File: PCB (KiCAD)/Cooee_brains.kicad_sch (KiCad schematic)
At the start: 36 parts, among them J1 USB4105-GF-A, J2 Conn_Coaxial, J3 503398-1892, J4 Conn_01x14_Socket, J5 Conn_01x02_Pin, J6 Conn_Coaxial, J7 Conn_01x04_Pin, J9 Conn_01x05_Socket, SW1 Prog, SW2 Reset, U1 AMS1117-3.3, U2 ESP32-S3-WROOM-1-N8, U3 MAX98357AETE_T, U6 INTERFACE-CP2102-GMR_QFN28_, U8 RA-01H

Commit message: more PCB work on the motherboard
more PCB work on the motherboard
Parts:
- added C5, C9: 4.7uF, Capacitor_SMD:C_0805_2012Metric, symbol Device:C_Small
- added C6, C8: 100nF, Capacitor_SMD:C_0805_2012Metric, symbol Device:C_Small
- added C7: 1uF, Capacitor_SMD:C_0805_2012Metric, symbol Device:C_Small
- added D1: D, Diode_SMD:D_0805_2012Metric_Pad1.15x1.40mm_HandSolder, symbol Device:D
- added H3: MountingHole_Pad_MP, MountingHole:MountingHole_3.2mm_M3_DIN965_Pad_TopBottom, symbol Mechanical:MountingHole_Pad_MP
- added JP1: SolderJumper_2_Open, Jumper:SolderJumper-2_P1.3mm_Open_RoundedPad1.0x1.5mm, symbol Jumper:SolderJumper_2_Open
- added R11, R12, R13, R14, R8: 10kΩ, Capacitor_SMD:C_0805_2012Metric_Pad1.18x1.45mm_HandSolder, symbol stormduino-Rev2-rescue:R-Device
- U5: value ~ -> M210Z
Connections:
- net BigSD_MISO is gone; now on net SHARED_MISO: J7.2 (Pin_2)
- net BigSD_MOSI is gone; now on net SHARED_MOSI: J7.3 (Pin_3)
- net BigSD_SCK is gone; now on net SHARED_CLCK: J7.1 (Pin_1)
- net SD_CLK is gone; now on net SHARED_CLCK: J3.5 (CLK)
- net SD_DAT0 is gone; now on net SHARED_MISO: J3.7 (DAT0)
- net 3.3V: now also J3.4 (VDD), MK1.7 (VDD), U5.14 (Vcc_RF), U5.8 (VCC), U6.6 (VDD), C8.2, C9.1, R11.1, R12.1
- net 5V: now also U6.7 (REGIN), U6.8 (VBUS), C6.1, C7.1, D1.2 (A); no longer C1.2, U1.3 (VI)
- net Batt+: now also C1.2, U1.3 (VI), D1.1 (K)
- net GND: now also C5.1, C6.2, C7.2, C8.1, C9.2, H3.MP, R13.1, R14.1, R8.1
- net KEEB_SCL: now also U2.10 (IO17); no longer U2.15 (IO3)
- net LoRa_Select: now also U2.25 (IO48); no longer U2.16 (IO46)
- net SHARED_CLCK: now also J4.10 (Pin_10), U8.12 (SCK)
- net SHARED_MISO: now also J4.13 (Pin_13), U8.13 (MISO)
- net SHARED_MOSI: now also J3.3 (CMD), J4.12 (Pin_12), U8.14 (MOSI)
- net SPEAKER+: now also J5.2 (Pin_2); no longer J5.1 (Pin_1)
- net SPEAKER-: now also J5.1 (Pin_1); no longer J5.2 (Pin_2)
- net T_CS: now also U2.8 (IO15); no longer U2.21 (IO13)
- net USB_D+: no longer U6.4 (D+)
- net USB_D-: no longer U6.5 (D-)
- net USB_DN: now also U6.5 (D-); no longer U2.13 (IO19)
- net USB_DP: now also U6.4 (D+); no longer U2.14 (IO20)
- net MIC_BCLK: now reaches U2.11 (IO18)
- net MIC_BCLK: now also MK1.1 (SCK)
- net MIC_EN: now reaches U2.23 (IO21)
- net MIC_EN: now also MK1.8 (CHIPEN)
- net GPS_RST: now reaches U2.32 (IO39)
- net GPS_RST: now also U5.9 (RST)
- net GPS_On/OFF: now reaches U2.33 (IO40)
- net GPS_On/OFF: now also U5.5 (On/Off)
- net GPS_SlaveIn: now reaches U2.34 (IO41)
- net GPS_SlaveIn: now also U5.3 (GPS_RxData)
- net GPS_SlaveOut: now reaches U2.35 (IO42)
- net GPS_SlaveOut: now also U5.2 (GPS_TxData)
- net Interface_Tx: now reaches U2.36 (RXD0)
- net Interface_Tx: now also U6.26 (TXD)
- net Interface_Rx: now reaches U2.37 (TXD0)
- net Interface_Rx: now also U6.25 (RXD)
- net SPKR_DIN: now reaches U3.1 (DIN)
- net SPKR_DIN: now also U2.21 (IO13)
- net SPKR_LRCK: now reaches U3.14 (LRCLK)
- net SPKR_LRCK: now also U2.22 (IO14)
- net SPKR_BCLK: now reaches U3.16 (BCLK)
- net SPKR_BCLK: now also U2.20 (IO12)
- net SPKR_EN: now reaches U3.17 (EP)
- net at U3.2 (GAIN_SLOT): now also R14.2
- net at U3.4 (SD_MODE): now also R13.2
- net MIC_DOUT: now reaches MK1.2 (SD)
- net MIC_DOUT: now also U2.14 (IO20)
- net MIC_LRCK: now reaches MK1.3 (WS)
- net MIC_LRCK: now also U2.13 (IO19)
- net at MK1.4 (L/R): now also R12.2
- net at U6.11 (~{SUSPEND}): now also R8.2
- net at U6.18 (NC/VPP): now also C5.2
- net at U6.9 (~{RST}): now also R11.2
- net MICRO_SD_CS: now reaches J3.2 (CD/DAT3^2)
- net KEEP_RST renamed KEEB_INT
- removed net LoRa_MISO: U2.25 (IO48), U8.13 (MISO)
- net LoRa_MOSI: no longer names the net of U2.24 (IO47)
- net LoRa_MOSI: no longer U8.14 (MOSI)
- net LoRa_SCLK: no longer names the net of U2.26 (IO45)
- net LoRa_SCLK: no longer U8.12 (SCK)
- removed net T_CLK: J4.10 (Pin_10), U2.20 (IO12)
- removed net T_MISO: J4.13 (Pin_13), U2.8 (IO15)
- removed net T_MOSI: J4.12 (Pin_12), U2.22 (IO14)
- no-connect marks 0 -> 5
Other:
- note added: "AUDIO"
- note added: "CONNECTORS"
- note added: "Check operating voltage"
- note added: "Clear To Send"
- note added: "Data Carrier Detect"
- note added: "Data Set Ready"
- note added: "Data Terminal Ready"
- note added: "Do any of these components need 5V? Can we skip boosting the battery and instead only buck to 3.3 from battery?"
- note added: "Does the interface need to be wired to GPIO0 to enable bootloader mode?"
- note added: "HXY 8205A -- MOSFET array"
- note added: "I2C not SPI"
- note added: "Investigate:"
- note added: "M210Z"
- note added: "MIC"
- note added: "Make some optional (solder bridge) lines that connect the USB directly to ESP32"
- note added: "POWER"
- note added: "QWERTY"
- note added: "Ready to Send"
- note added: "SIGNAL"
- note added: "So that we don't need the interface chip (or if it breaks or whatever)"
- note added: "The ESP32 can only have TWO(2) SPI busses"
- note added: "XBLW TP4056EDTR(XBLW) --charging IC"
- note removed: "Max out at 4V regardless of type?"
- note removed: "Needs to support either NaIon or LiIon!"
- note removed: "USB"
- moved on the sheet: C1, C2, C3, C4, D72, D73, D74, J1, J2, J3, J4, J5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

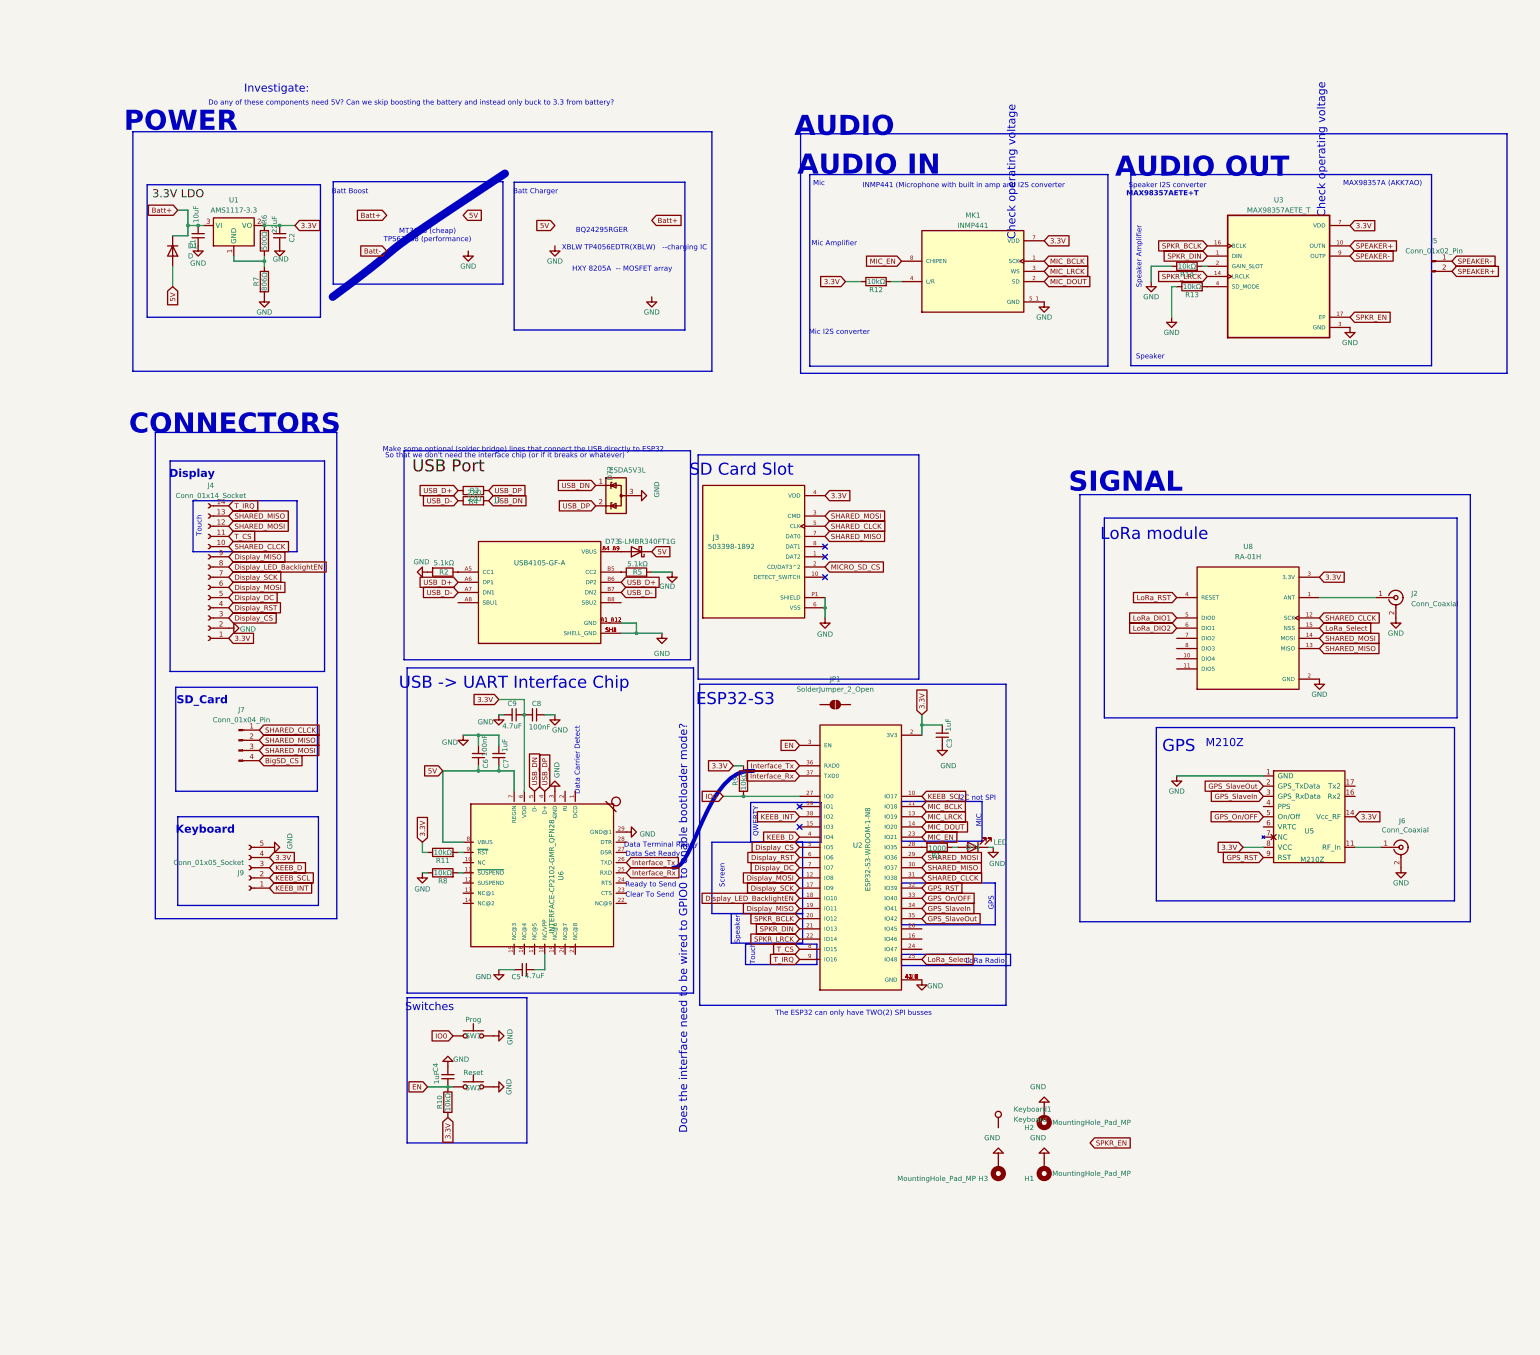
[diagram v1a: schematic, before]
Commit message: motherboard PCB work
motherboard PCB work
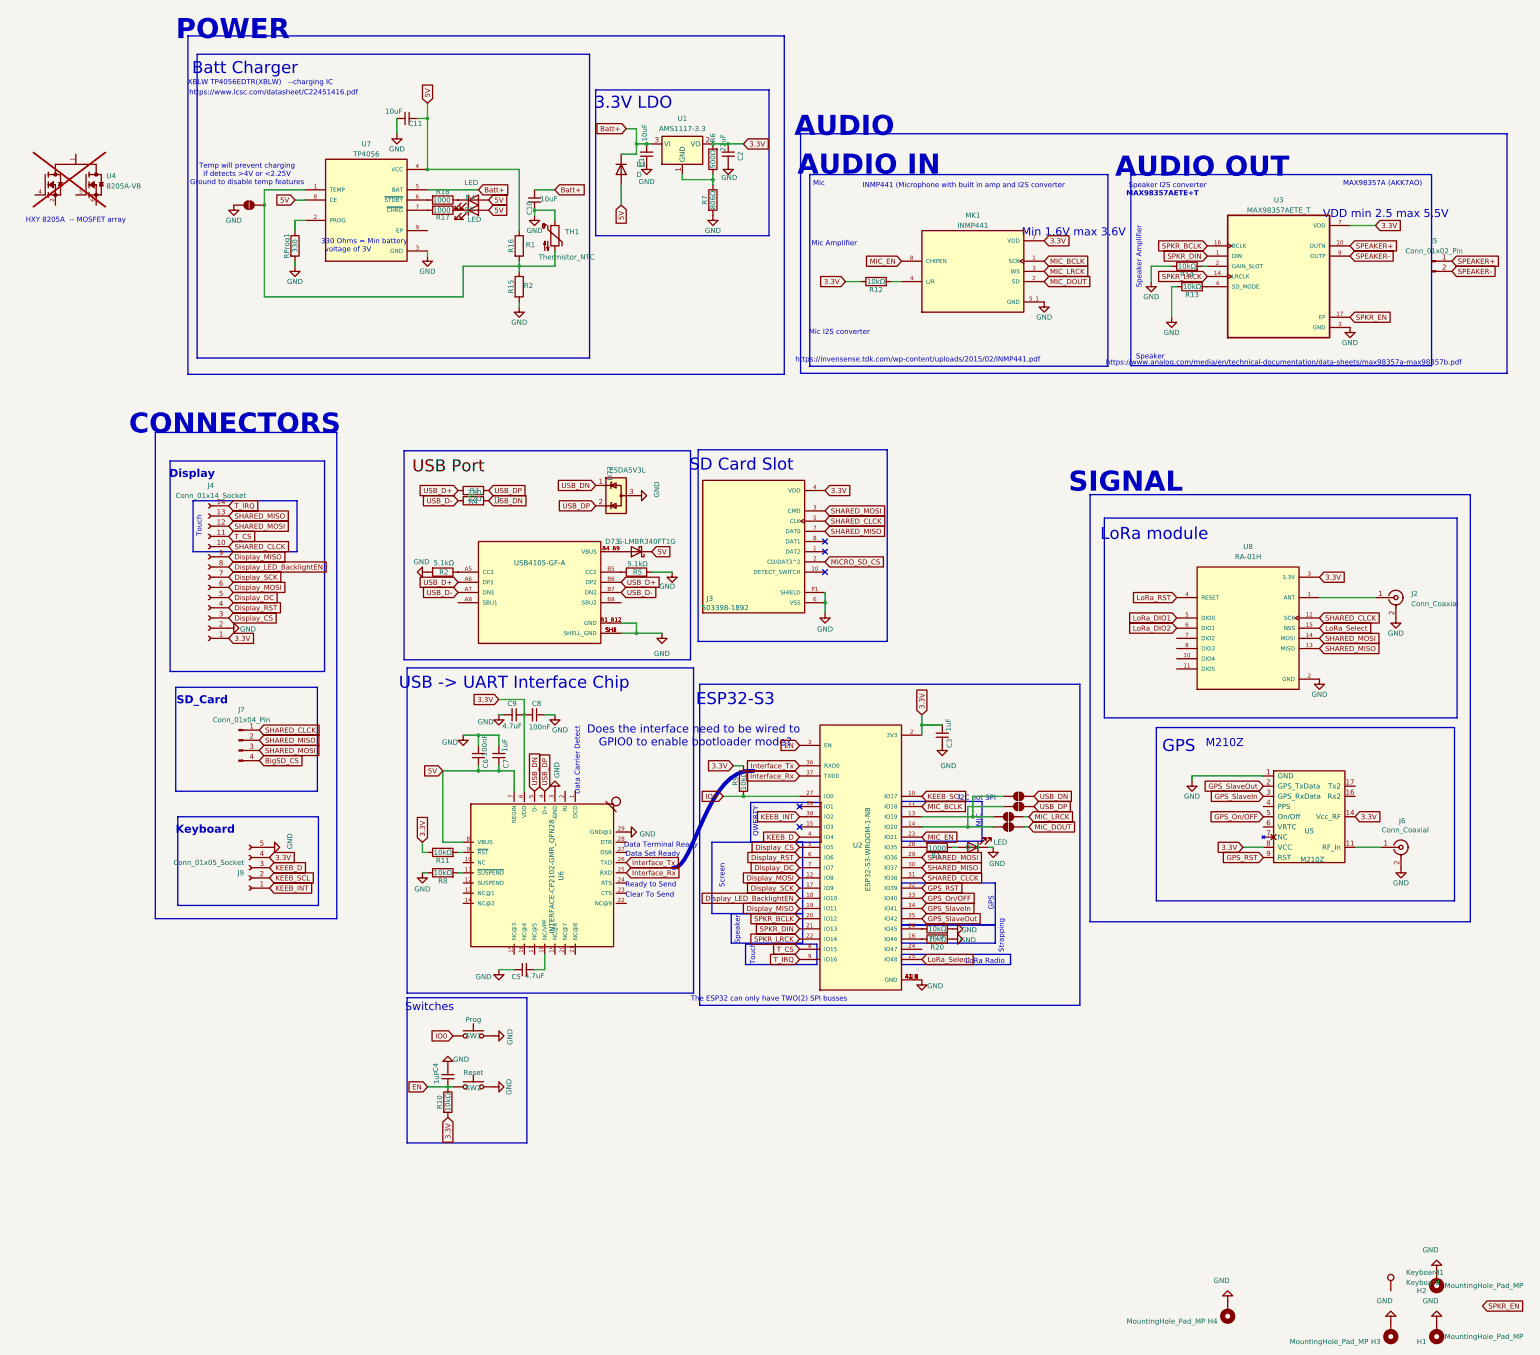
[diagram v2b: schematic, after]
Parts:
- added C10, C11: 10uF, Capacitor_SMD:C_0805_2012Metric, symbol Device:C_Small
- added D4, D5: LED, Capacitor_SMD:C_0805_2012Metric, symbol Device:LED
- added H4: MountingHole_Pad_MP, MountingHole:MountingHole_3.2mm_M3_DIN965_Pad_TopBottom, symbol Mechanical:MountingHole_Pad_MP
- added JP2, JP3, JP4, JP5: SolderJumper_2_Open, Jumper:SolderJumper-2_P1.3mm_Open_RoundedPad1.0x1.5mm, symbol Jumper:SolderJumper_2_Open
- added R15: R2, Capacitor_SMD:C_0805_2012Metric_Pad1.18x1.45mm_HandSolder, symbol stormduino-Rev2-rescue:R-Device
- added R16: R1, Capacitor_SMD:C_0805_2012Metric_Pad1.18x1.45mm_HandSolder, symbol stormduino-Rev2-rescue:R-Device
- added R17, R18: 1000, Capacitor_SMD:C_0805_2012Metric_Pad1.18x1.45mm_HandSolder, symbol stormduino-Rev2-rescue:R-Device
- added R19, R20: 10kΩ, Capacitor_SMD:C_0805_2012Metric_Pad1.18x1.45mm_HandSolder, symbol stormduino-Rev2-rescue:R-Device
- added RProg1: 330, Capacitor_SMD:C_0805_2012Metric_Pad1.18x1.45mm_HandSolder, symbol stormduino-Rev2-rescue:R-Device
- added TH1: Thermistor_NTC, Resistor_SMD:R_0805_2012Metric_Pad1.20x1.40mm_HandSolder, symbol Device:Thermistor_NTC
- added U4: 8205A-VB, USB4105-GF-A (1):SOP65P640X120-8N, symbol Downloaded:8205A-VB
- added U7: TP4056, USB4105-GF-A (1):SOP127P600X175-9N, symbol Downloaded:TP4056
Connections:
- net 3.3V is gone; now on net VDD: C2.2, C3.2, C8.2, C9.1, J3.4 (VDD), J4.1 (Pin_1), J9.4 (Pin_4), MK1.7 (VDD), R10.2, R11.1, R12.1, R6.2, R9.1, U1.2 (VO), U2.2 (3V3), U5.14 (Vcc_RF), U5.8 (VCC), U6.6 (VDD), U8.3 (3.3V)
- net 5V: now also C11.1, D4.2 (A), D5.2 (A), R16.1, U7.4 (VCC), U7.8 (CE)
- net Batt+: now also C10.2, U7.5 (BAT)
- net GND: now also C10.1, C11.2, H4.MP, JP5.1 (A), R15.2, R19.2, R20.2, RProg1.2, TH1.1, U7.3 (GND)
- net MIC_DOUT: now also JP4.2 (B); no longer U2.14 (IO20)
- net MIC_LRCK: now also JP3.2 (B); no longer U2.13 (IO19)
- net SPEAKER+: now also J5.1 (Pin_1); no longer J5.2 (Pin_2)
- net SPEAKER-: now also J5.2 (Pin_2); no longer J5.1 (Pin_1)
- net USB_DN: now also JP1.2 (B)
- net USB_DP: now also JP2.2 (B)
- net at U2.16 (IO46): now also R20.1
- net at U2.26 (IO45): now also R19.1
- net at JP1.1 (A): now also U2.13 (IO19), JP3.1 (A)
- new net: JP2.1 (A), JP4.1 (A), U2.14 (IO20)
- new net: D4.1 (K), R18.1
- new net: JP5.2 (B), R15.1, R16.2, TH1.2, U7.1 (TEMP)
- new net: D5.1 (K), R17.1
- new net: R18.2, U7.6 (~{STDBY})
- new net: U4.1, U4.8
- new net: U4.2, U4.3
- new net: U4.6, U4.7
- new net: RProg1.1, U7.2 (PROG)
- new net: R17.2, U7.7 (~{CHRG})
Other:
- note added: "3.3V LDO"
- note added: "330 Ohms = Min battery"
- note added: "Min 1.6V max 3.6V"
- note added: "Strapping"
- note added: "Temp will prevent charging if detects >4V or <2.25V Ground to disable temp features"
- note added: "VDD min 2.5 max 5.5V"
- note added: "https://invensense.tdk.com/wp-content/uploads/2015/02/INMP441.pdf"
- note added: "https://www.analog.com/media/en/technical-documentation/data-sheets/max98357a-max98357b.pdf"
- note added: "https://www.lcsc.com/datasheet/C22451416.pdf"
- note added: "voltage of 3V"
- note removed: "BQ24295RGER"
- note removed: "Batt Boost"
- note removed: "Check operating voltage"
- note removed: "Do any of these components need 5V? Can we skip boosting the battery and instead only buck to 3.3 from battery?"
- note removed: "Investigate:"
- note removed: "MT3608 (cheap) TPS61088 (performance)"
- note removed: "Make some optional (solder bridge) lines that connect the USB directly to ESP32"
- note removed: "So that we don't need the interface chip (or if it breaks or whatever)"
- moved on the sheet: C1, C2, D1, H1, H2, H3, J3, Keyboard1, R6, R7, U1

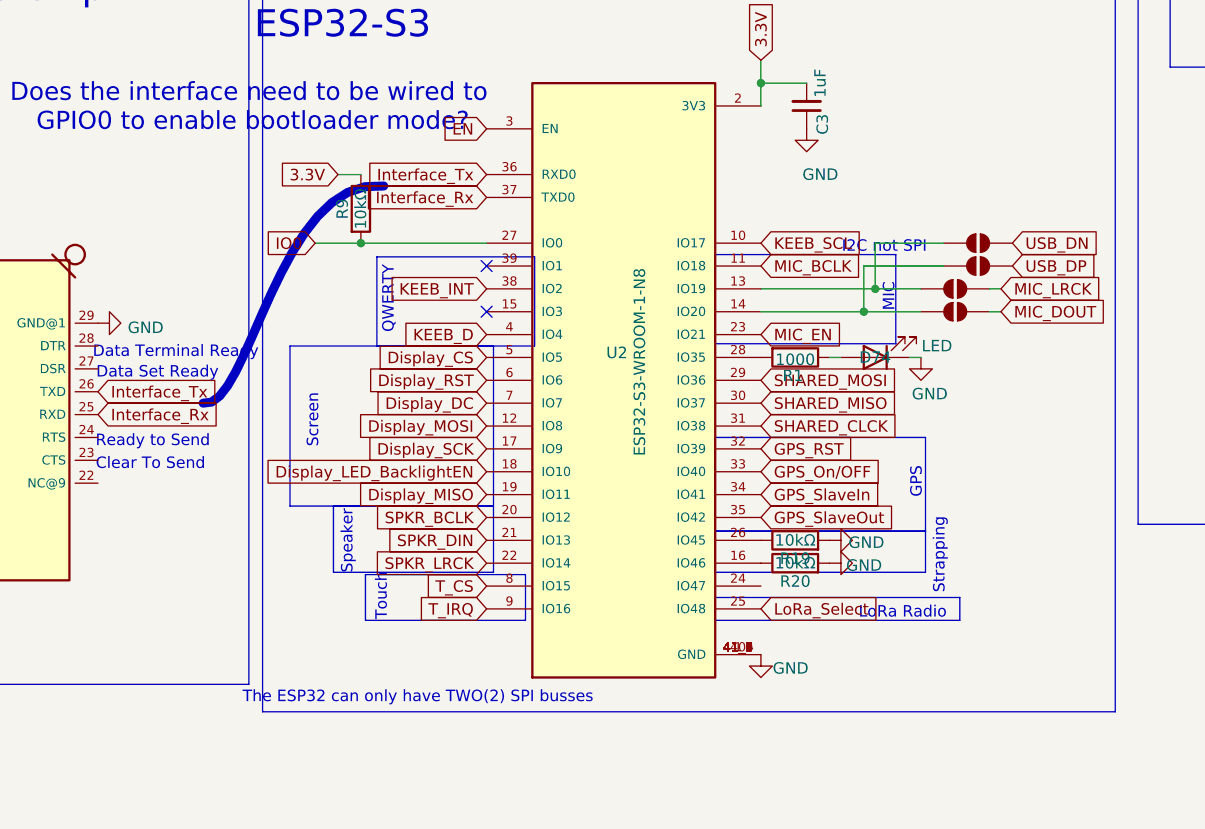
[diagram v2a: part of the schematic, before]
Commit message: trying to figure out the dang i2s device configurations
trying to figure out the dang i2s device configurations
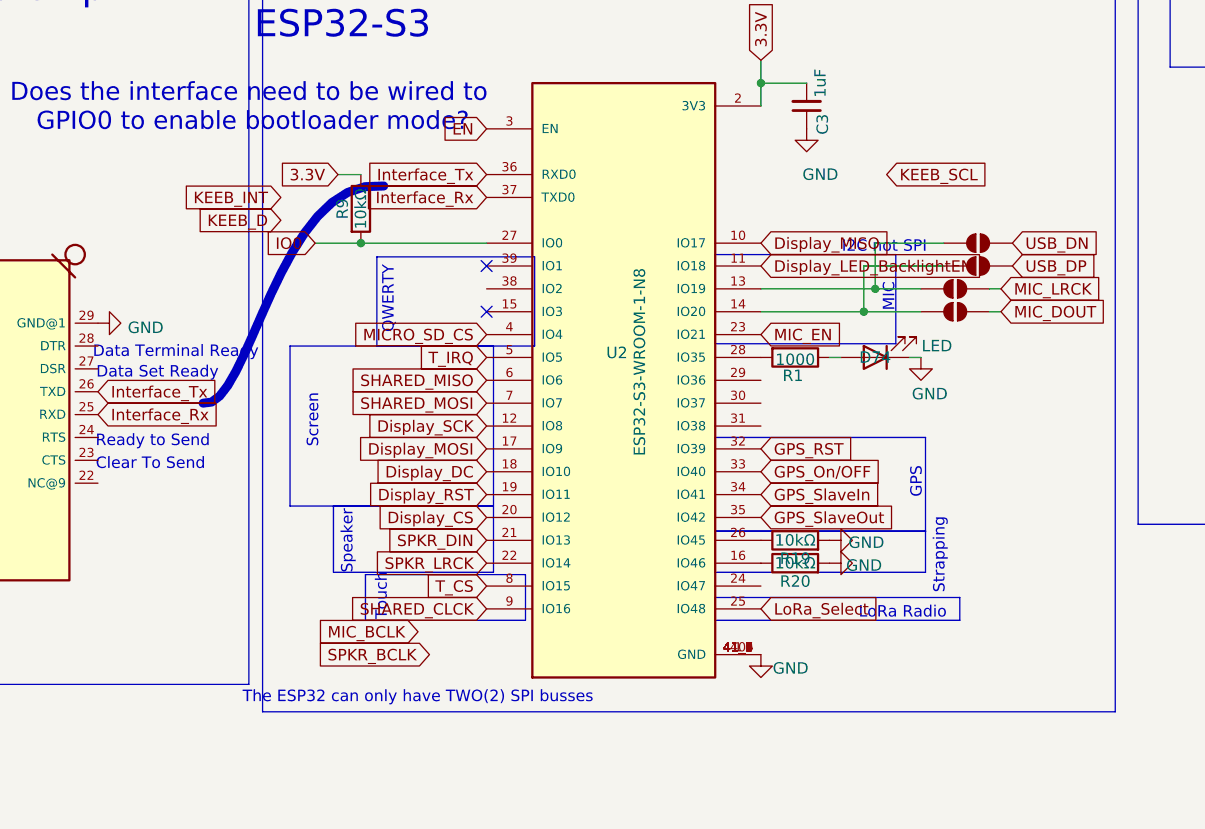
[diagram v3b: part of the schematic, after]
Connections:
- net Display_CS: now also U2.20 (IO12); no longer U2.5 (IO5)
- net Display_DC: now also U2.18 (IO10); no longer U2.7 (IO7)
- net Display_LED_BacklightEN: now also U2.11 (IO18); no longer U2.18 (IO10)
- net Display_MISO: now also U2.10 (IO17); no longer U2.19 (IO11)
- net Display_MOSI: now also U2.17 (IO9); no longer U2.12 (IO8)
- net Display_RST: now also U2.19 (IO11); no longer U2.6 (IO6)
- net Display_SCK: now also U2.12 (IO8); no longer U2.17 (IO9)
- net KEEB_D: no longer U2.4 (IO4)
- net KEEB_INT: no longer U2.38 (IO2)
- net KEEB_SCL: no longer U2.10 (IO17)
- net MICRO_SD_CS: now also U2.4 (IO4)
- net MIC_BCLK: no longer U2.11 (IO18)
- net SHARED_CLCK: now also U2.9 (IO16); no longer U2.31 (IO38)
- net SHARED_MISO: now also U2.6 (IO6); no longer U2.30 (IO37)
- net SHARED_MOSI: now also U2.7 (IO7); no longer U2.29 (IO36)
- net SPKR_BCLK: no longer U2.20 (IO12)
- net T_IRQ: now also U2.5 (IO5); no longer U2.9 (IO16)
